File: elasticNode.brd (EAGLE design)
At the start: 58.2 x 52.5 mm, 135 parts, among them J1 FEMALE_HEADER_2X1, J2 JUMPER, J3 JUMPER, J5 FEMALE_HEADER_10X2, J6 USB_CONNMICRO_SMT, J7 USB_CONNMICRO_SMT, M1 SISS23DN, M2 SISS23DN, M3 SISS23DN, M4 SISS23DN, U1 AT90USB128, U10 LTC3419DFN, U11 PAC1720, U14 LTC3419DFN, U2 IS66WV51216EALL, U3 MRF24J40MA, U4 SPARTAN7-LX15, U5 ATMEGA32U4QFN, U6 SST26VF032BWDFN, U7 PAC1720, U8 PAC1720, U9 PAC1720, X1 8MHz, X2 50MHz, X3 32MHz, X4 100MHz, X5 8MHz

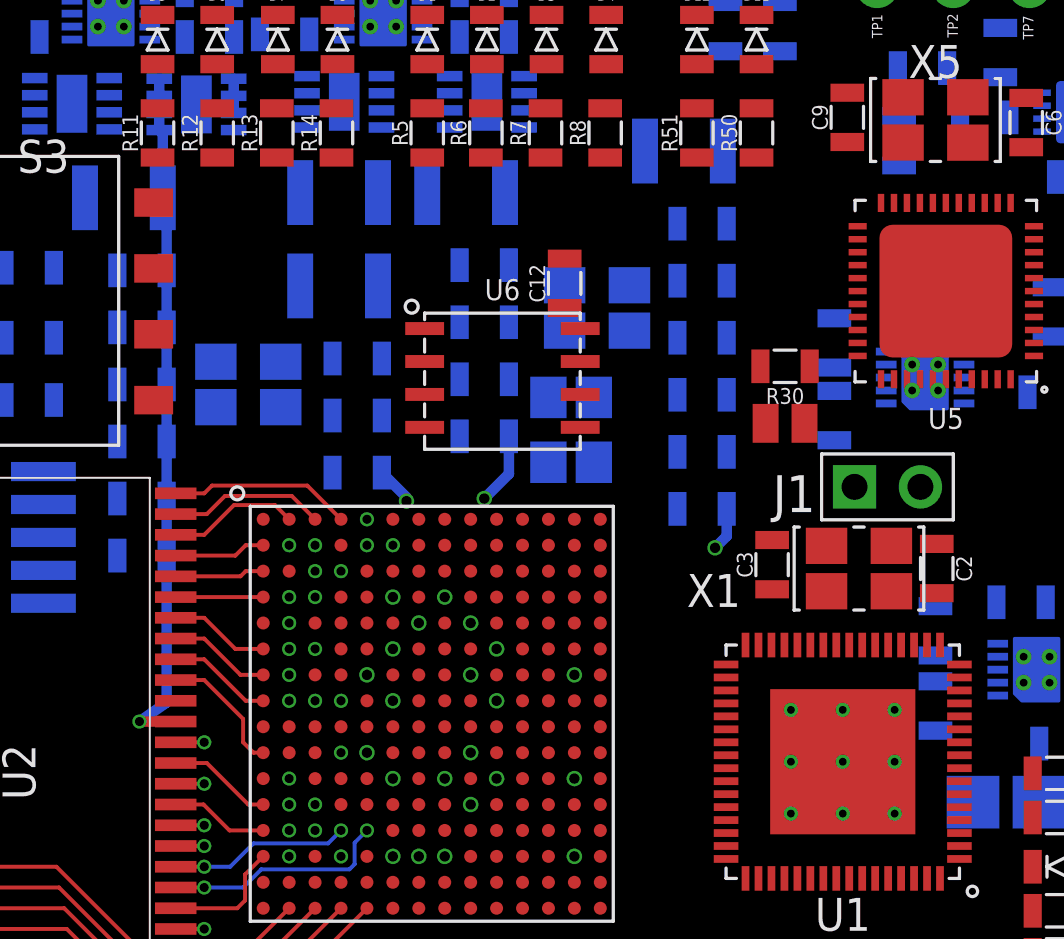
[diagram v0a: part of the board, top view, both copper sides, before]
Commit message: back up
spi_sck didn’t connect to FPGA,OK？
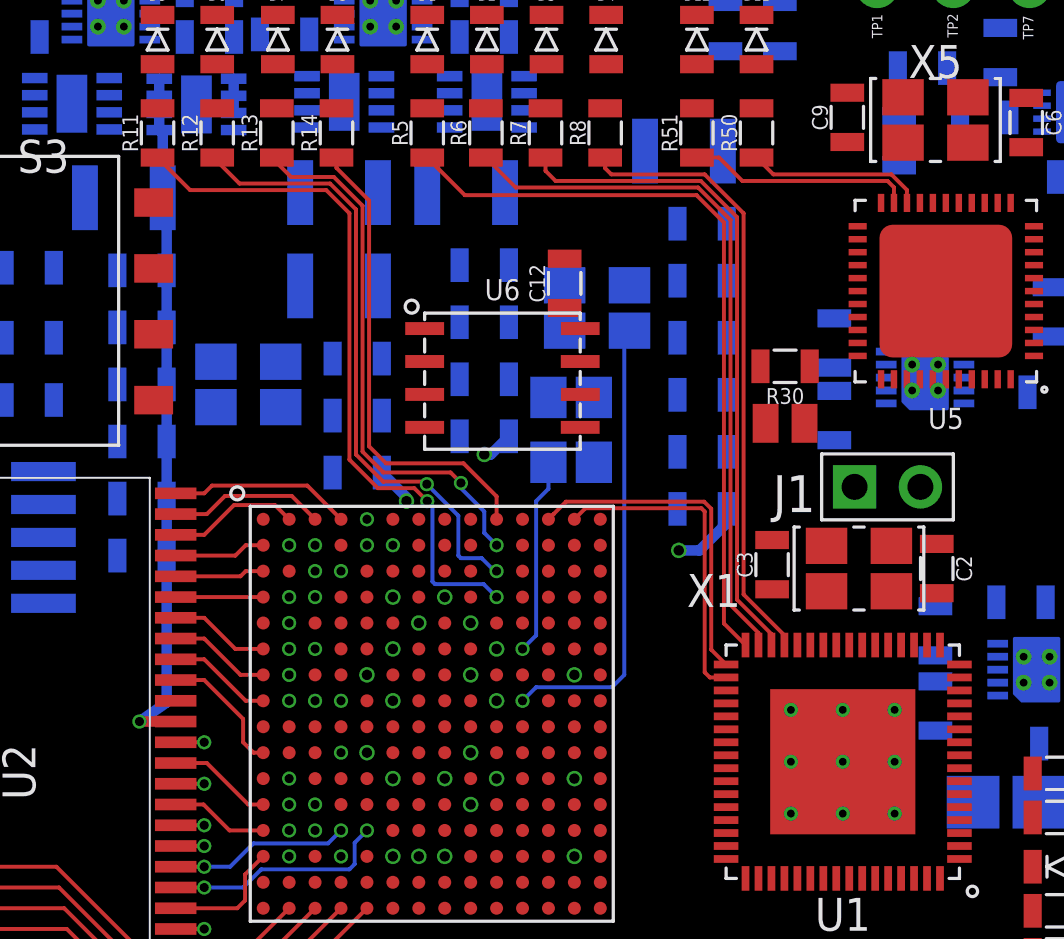
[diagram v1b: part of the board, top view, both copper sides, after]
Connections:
- net AD6/SELECTMAP_D1/SPI_MISO/MCU_PDO: now also U4.B12
- net AD7/SELECTMAP_D0/SPI_MOSI/PDI: now also U4.B11
- net FPGA_LED0: now also U4.D10
- net FPGA_LED1: now also U4.C10
- net FPGA_LED2: now also U4.B10
- net FPGA_LED3: now also U4.A10
- net XMEM_A10: no longer U4.B13
- net XMEM_A12: no longer U4.C12, U4.C14
- net XMEM_A13: no longer U4.D12
- net XMEM_A8: no longer U4.B12
- net XMEM_A9: no longer U4.B14
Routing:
- net MCU_LED0: track 0.00 -> 29.1 mm
- net FPGA_LED0: track 0.00 -> 27.4 mm, vias 0 -> 2
- net MCU_LED1: track 0.00 -> 27.3 mm
- net MCU_LED2: track 0.00 -> 25.7 mm
- net FPGA_LED1: track 0.00 -> 23.9 mm, vias 0 -> 2
- net MCU_LED3: track 0.00 -> 23.8 mm
- net FPGA_LED2: track 0.00 -> 20.9 mm, vias 0 -> 2
- net FPGA_LED3: track 0.00 -> 18.3 mm
- net OSC_32: track 0.00 -> 17.7 mm, vias 0 -> 1
- net XMEM_WR: track 0.00 -> 12.9 mm
- net XMEM_RD: track 0.00 -> 12.4 mm
- net MON_LED1: track 0.00 -> 8.68 mm
- net OSC_50: track 0.00 -> 7.61 mm, vias 0 -> 1
- net MON_LED0: track 0.00 -> 6.82 mm
